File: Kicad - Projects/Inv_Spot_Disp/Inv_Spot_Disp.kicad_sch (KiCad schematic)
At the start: 43 parts, among them J1 PWM_Out, J2 Power_Supply, J3 Current_Sense, J4 Prog, J6 Temp_Sense, SW1 1, SW2 2, SW3 3, SW4 4, SW5 SW_Push, U1 STM32F030F4Px, U2 LCD-016N002L, U3 AMS1117-3.3, U4 LKS561, U5 LM358, U6 LTV-817S

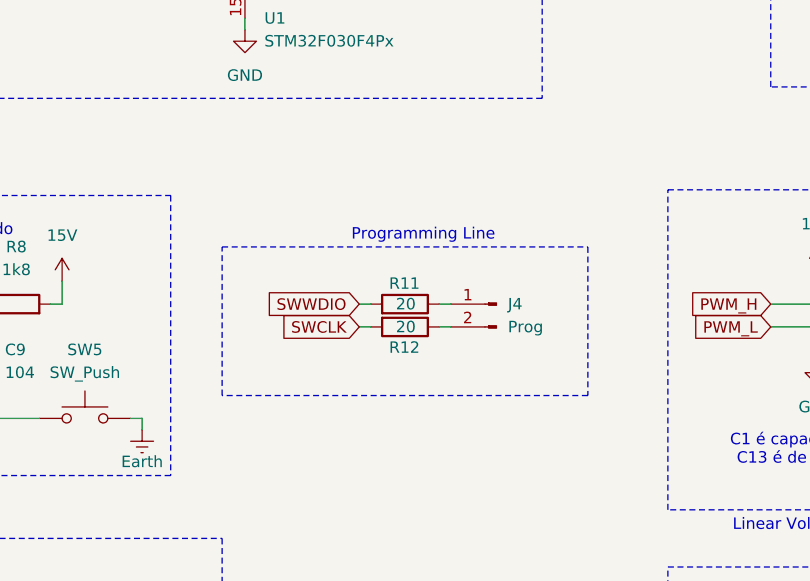
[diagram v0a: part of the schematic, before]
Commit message: Ajustes Gerais
Ajustes Gerais
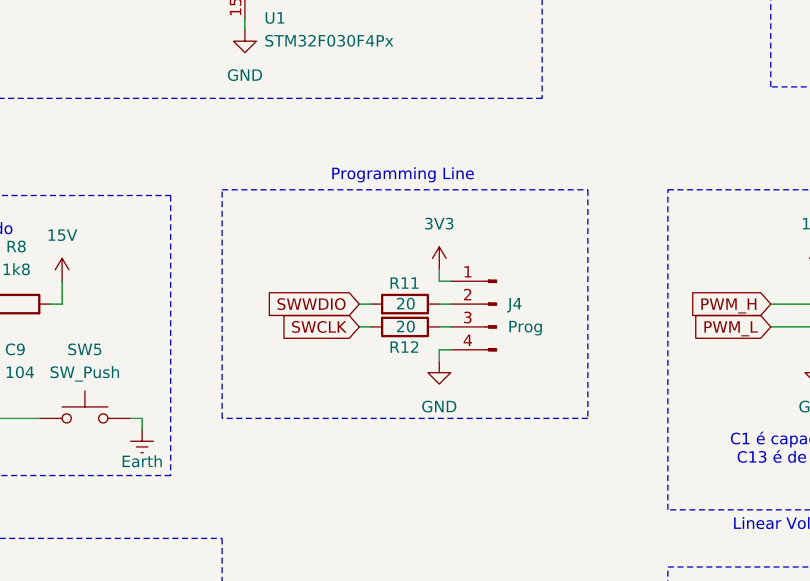
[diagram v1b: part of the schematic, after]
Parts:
- removed J4: Prog, Connector_PinHeader_2.00mm:PinHeader_1x02_P2.00mm_Vertical, symbol Connector:Conn_01x02_Pin
- added J4: Prog, Connector_PinHeader_2.00mm:PinHeader_1x04_P2.00mm_Vertical, symbol Connector:Conn_01x04_Pin
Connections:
- net 3V3: now also J4.1 (Pin_1)
- net GND: now also J4.4 (Pin_4)
- net at R11.1: now also J4.2 (Pin_2)
- net at R12.1: now also J4.3 (Pin_3)
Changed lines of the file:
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@@
 	)
 	(rectangle
-		(start 128.27 99.06)
-		(end 168.91 115.57)
+		(start 128.27 92.71)
+		(end 168.91 118.11)
 		(stroke
 			(width 0)
@@
 	(text "Programming Line"
 		(exclude_from_sim no)
-		(at 150.622 97.79 0)
+		(at 148.336 91.186 0)
 		(effects
 			(font
@@
 	(wire
 		(pts
+			(xy 153.67 102.87) (xy 152.4 102.87)
+		)
+		(stroke
+			(width 0)
+			(type default)
+		)
+	)
+	(wire
+		(pts
 			(xy 73.66 39.37) (xy 73.66 41.91)
 		)
@@
 	(wire
 		(pts
+			(xy 152.4 102.87) (xy 152.4 101.6)
+		)
+		(stroke
+			(width 0)
+			(type default)
+		)
+	)
+	(wire
+		(pts
 			(xy 146.05 66.04) (xy 143.51 66.04)
 		)
@@
 	(wire
 		(pts
+			(xy 153.67 110.49) (xy 152.4 110.49)
+		)
+		(stroke
+			(width 0)
+			(type default)
+		)
+	)
+	(wire
+		(pts
 			(xy 64.77 168.91) (xy 64.77 172.72)
 		)
@@
 	(wire
 		(pts
+			(xy 152.4 110.49) (xy 152.4 111.76)
+		)
+		(stroke
+			(width 0)
+			(type default)
+		)
+	)
+	(wire
+		(pts
 			(xy 273.05 105.41) (xy 273.05 109.22)
 		)
@@
 	)
 	(symbol
-		(lib_id "Connector:Conn_01x02_Pin")
-		(at 158.75 105.41 0)
-		(mirror y)
-		(unit 1)
-		(body_style 1)
-		(exclude_from_sim no)
-		(in_bom yes)
-		(on_board yes)
-		(in_pos_files yes)
-		(dnp no)
-		(fields_autoplaced yes)
-		(property "Reference" "J4"
-			(at 160.02 105.4099 0)
-			(show_name no)
-			(do_not_autoplace no)
-			(effects
-				(font
-					(size 1.27 1.27)
-				)
-				(justify right)
-			)
-		)
-		(property "Value" "Prog"
-			(at 160.02 107.9499 0)
-			(show_name no)
-			(do_not_autoplace no)
-			(effects
-				(font
-					(size 1.27 1.27)
-				)
-				(justify right)
-			)
-		)
-		(property "Footprint" "Connector_PinHeader_2.00mm:PinHeader_1x02_P2.00mm_Vertical"
-			(at 158.75 105.41 0)
-			(hide yes)
-			(show_name no)
-			(do_not_autoplace no)
-			(effects
-				(font
-					(size 1.27 1.27)
-				)
-			)
-		)
-		(property "Datasheet" ""
-			(at 158.75 105.41 0)
-			(hide yes)
-			(show_name no)
-			(do_not_autoplace no)
-			(effects
-				(font
-					(size 1.27 1.27)
-				)
-			)
-		)
-		(property "Description" "Generic connector, single row, 01x02, script generated"
-			(at 158.75 105.41 0)
-			(hide yes)
-			(show_name no)
-			(do_not_autoplace no)
-			(effects
-				(font
-					(size 1.27 1.27)
-				)
-			)
-		)
-		(pin "1"
-		)
-		(pin "2"
-		)
-		(instances
-			(project "Inv_Spot_Disp"
-				(path "/016976b8-e488-405d-b5a2-1b3e7431e7ce"
-					(reference "J4")
-					(unit 1)
-				)
-			)
-		)
-	)
-	(symbol
 		(lib_id "power:VCC")
 		(at 232.41 30.48 0)
@@
 	)
 	(symbol
+		(lib_id "power:VCC")
+		(at 152.4 101.6 0)
+		(unit 1)
+		(body_style 1)
+		(exclude_from_sim no)
+		(in_bom yes)
+		(on_board yes)
+		(in_pos_files yes)
+		(dnp no)
+		(fields_autoplaced yes)
+		(property "Reference" "#PWR023"
+			(at 152.4 105.41 0)
+			(hide yes)
+			(show_name no)
+			(do_not_autoplace no)
+			(effects
+				(font
+					(size 1.27 1.27)
+				)
+			)
+		)
+		(property "Value" "3V3"
+			(at 152.4 96.52 0)
+			(show_name no)
+			(do_not_autoplace no)
+			(effects
+				(font
+					(size 1.27 1.27)
+				)
+			)
+		)
+		(property "Footprint" ""
+			(at 152.4 101.6 0)
+			(hide yes)
+			(show_name no)
+			(do_not_autoplace no)
+			(effects
+				(font
+					(size 1.27 1.27)
+				)
+			)
+		)
+		(property "Datasheet" ""
+			(at 152.4 101.6 0)
+			(hide yes)
+			(show_name no)
+			(do_not_autoplace no)
+			(effects
+				(font
+					(size 1.27 1.27)
+				)
+			)
+		)
+		(property "Description" "Power symbol creates a global label with name \"VCC\""
+			(at 152.4 101.6 0)
+			(hide yes)
+			(show_name no)
+			(do_not_autoplace no)
+			(effects
+				(font
+					(size 1.27 1.27)
+				)
+			)
+		)
+		(pin "1"
+		)
+		(instances
+			(project "Inv_Spot_Disp"
+				(path "/016976b8-e488-405d-b5a2-1b3e7431e7ce"
+					(reference "#PWR023")
+					(unit 1)
+				)
+			)
+		)
+	)
+	(symbol
 		(lib_id "power:GND")
 		(at 29.21 63.5 0)
@@
 	)
 	(symbol
+		(lib_id "power:GND")
+		(at 152.4 111.76 0)
+		(unit 1)
+		(body_style 1)
+		(exclude_from_sim no)
+		(in_bom yes)
+		(on_board yes)
+		(in_pos_files yes)
+		(dnp no)
+		(fields_autoplaced yes)
+		(property "Reference" "#PWR022"
+			(at 152.4 118.11 0)
+			(hide yes)
+			(show_name no)
+			(do_not_autoplace no)
+			(effects
+				(font
+					(size 1.27 1.27)
+				)
+			)
+		)
+		(property "Value" "GND"
+			(at 152.4 116.84 0)
+			(show_name no)
+			(do_not_autoplace no)
+			(effects
+				(font
+					(size 1.27 1.27)
+				)
+			)
+		)
+		(property "Footprint" ""
+			(at 152.4 111.76 0)
+			(hide yes)
+			(show_name no)
+			(do_not_autoplace no)
+			(effects
+				(font
+					(size 1.27 1.27)
+				)
+			)
+		)
+		(property "Datasheet" ""
+			(at 152.4 111.76 0)
+			(hide yes)
+			(show_name no)
+			(do_not_autoplace no)
+			(effects
+				(font
+					(size 1.27 1.27)
+				)
+			)
+		)
+		(property "Description" "Power symbol creates a global label with name \"GND\" , ground"
+			(at 152.4 111.76 0)
+			(hide yes)
+			(show_name no)
+			(do_not_autoplace no)
+			(effects
+				(font
+					(size 1.27 1.27)
+				)
+			)
+		)
+		(pin "1"
+		)
+		(instances
+			(project "Inv_Spot_Disp"
+				(path "/016976b8-e488-405d-b5a2-1b3e7431e7ce"
+					(reference "#PWR022")
+					(unit 1)
+				)
+			)
+		)
+	)
+	(symbol
 		(lib_id "Device:C")
 		(at 120.65 168.91 0)
@@
 					(unit 1)
 				)
+			)
+		)
+	)
+	(symbol
+		(lib_id "Connector:Conn_01x04_Pin")
+		(at 158.75 105.41 0)
+		(mirror y)
+		(unit 1)
+		(body_style 1)
+		(exclude_from_sim no)
+		(in_bom yes)
+		(on_board yes)
+		(in_pos_files yes)
+		(dnp no)
+		(fields_autoplaced yes)
+		(property "Reference" "J4"
+			(at 160.02 105.4099 0)
+			(show_name no)
+			(do_not_autoplace no)
+			(effects
+				(font
+					(size 1.27 1.27)
+				)
+				(justify right)
+			)
+		)
+		(property "Value" "Prog"
+			(at 160.02 107.9499 0)
+			(show_name no)
+			(do_not_autoplace no)
+			(effects
+				(font
+					(size 1.27 1.27)
+				)
+				(justify right)
+			)
+		)
+		(property "Footprint" "Connector_PinHeader_2.00mm:PinHeader_1x04_P2.00mm_Vertical"
+			(at 158.75 105.41 0)
+			(hide yes)
+			(show_name no)
+			(do_not_autoplace no)
+			(effects
+				(font
+					(size 1.27 1.27)
+				)
+			)
+		)
+		(property "Datasheet" ""
+			(at 158.75 105.41 0)
+			(hide yes)
+			(show_name no)
+			(do_not_autoplace no)
+			(effects
+				(font
+					(size 1.27 1.27)
+				)
+			)
+		)
+		(property "Description" "Generic connector, single row, 01x04, script generated"
+			(at 158.75 105.41 0)
+			(hide yes)
+			(show_name no)
+			(do_not_autoplace no)
+			(effects
+				(font
+					(size 1.27 1.27)
+				)
+			)
+		)
+		(pin "1"
+		)
+		(pin "4"
+		)
+		(pin "2"
+		)
+		(pin "3"
+		)
+		(instances
+			(project "Inv_Spot_Disp"
+				(path "/016976b8-e488-405d-b5a2-1b3e7431e7ce"
+					(reference "J4")
+					(unit 1)
+				)
